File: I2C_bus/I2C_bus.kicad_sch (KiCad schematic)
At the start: 1 part, among them U1 ME6211C33M5

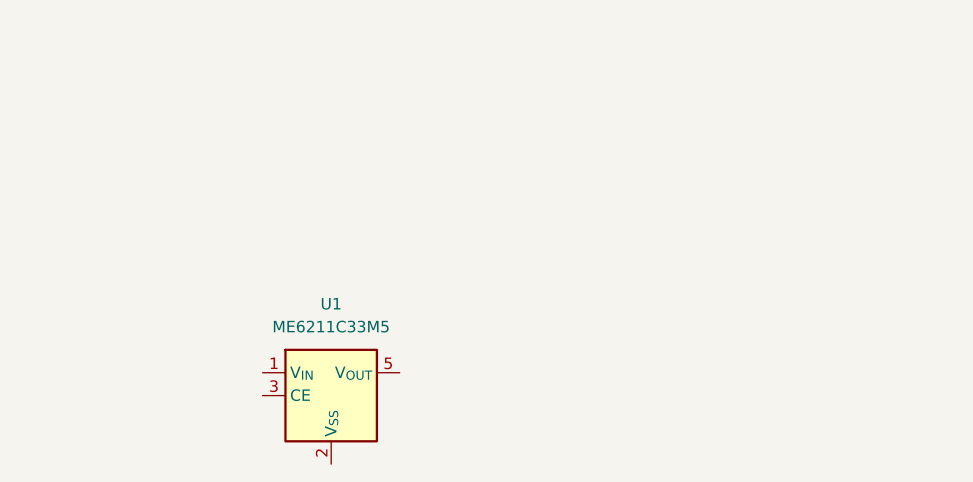
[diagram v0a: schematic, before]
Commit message: 繼續編輯
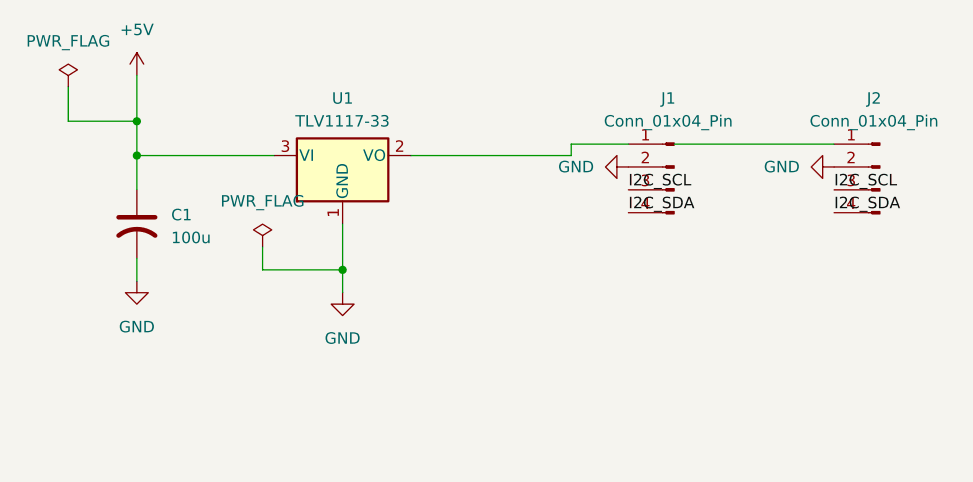
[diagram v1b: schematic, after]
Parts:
- removed U1: ME6211C33M5, Package_TO_SOT_SMD:SOT-23-5, symbol Regulator_Linear:ME6211C33M5
- added C1: 100u, Capacitor_SMD:C_0805_2012Metric_Pad1.18x1.45mm_HandSolder, symbol Device:C_US
- added J1, J2: Conn_01x04_Pin, symbol Connector:Conn_01x04_Pin
- added U1: TLV1117-33, symbol Regulator_Linear:TLV1117-33
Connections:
- new net: J1.1 (Pin_1), U1.2 (VO)
- new net +5V: C1.1, U1.3 (VI)
- new net GND: C1.2, J1.2 (Pin_2), J2.2 (Pin_2), U1.1 (GND)
- new net I2C_SCL: J1.3 (Pin_3), J2.3 (Pin_3)
- new net I2C_SDA: J1.4 (Pin_4), J2.4 (Pin_4)
